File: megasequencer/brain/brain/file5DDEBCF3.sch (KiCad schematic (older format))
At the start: 4 parts

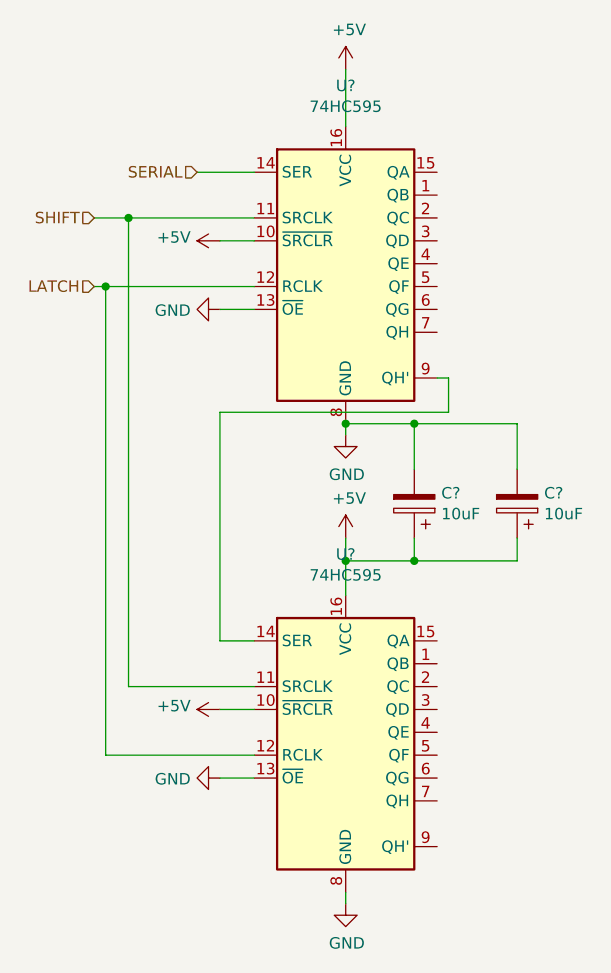
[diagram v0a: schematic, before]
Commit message: Fiddling with PCB a bit
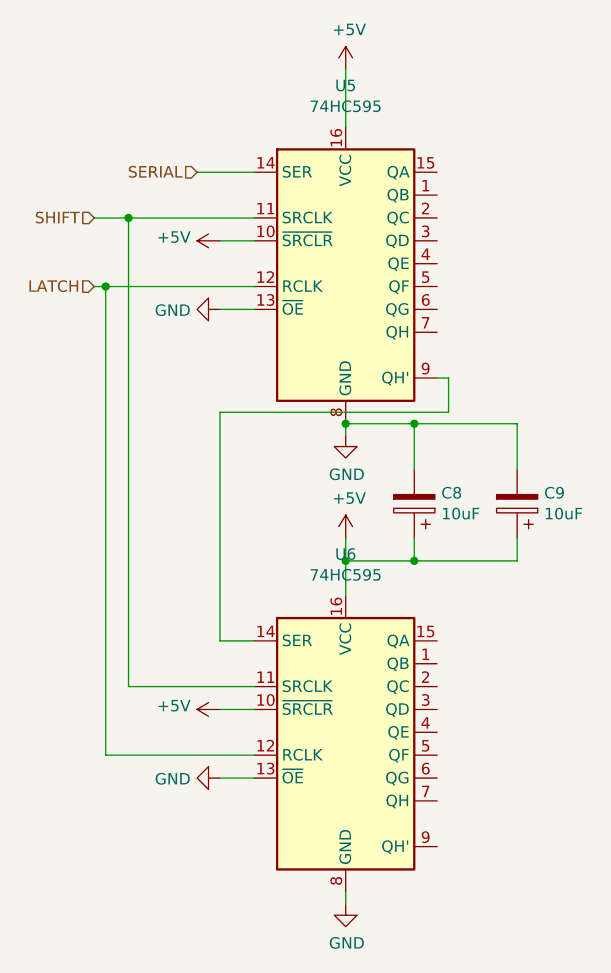
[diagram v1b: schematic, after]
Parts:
- gave numbers to parts that had none: 4
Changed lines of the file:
@@
 $EndDescr
 $Comp
-L power:+5V #PWR?
+L power:+5V #PWR0101
 U 1 1 5DDEC4E8
 P 2300 2150
-F 0 "#PWR?" H 2300 2000 50  0001 C CNN
+F 0 "#PWR0101" H 2300 2000 50  0001 C CNN
 F 1 "+5V" H 2315 2323 50  0000 C CNN
 F 2 "" H 2300 2150 50  0001 C CNN
@@
 $EndComp
 $Comp
-L 74xx:74HC595 U?
+L 74xx:74HC595 U5
 U 1 1 5DDEC62E
 P 2300 3000
-F 0 "U?" H 2300 3778 50  0000 C CNN
+F 0 "U5" H 2300 3778 50  0000 C CNN
 F 1 "74HC595" H 2300 3687 50  0000 C CNN
 F 2 "Package_DIP:DIP-16_W7.62mm" H 2300 3000 50  0001 C CNN
@@
 $EndComp
 $Comp
-L 74xx:74HC595 U?
+L 74xx:74HC595 U6
 U 1 1 5DDEC733
 P 2300 5050
-F 0 "U?" H 2300 5828 50  0000 C CNN
+F 0 "U6" H 2300 5828 50  0000 C CNN
 F 1 "74HC595" H 2300 5737 50  0000 C CNN
 F 2 "Package_DIP:DIP-16_W7.62mm" H 2300 5050 50  0001 C CNN
@@
 	2300 2150 2300 2400
 $Comp
-L power:+5V #PWR?
+L power:+5V #PWR0102
 U 1 1 5DDEC7AF
 P 2300 4200
-F 0 "#PWR?" H 2300 4050 50  0001 C CNN
+F 0 "#PWR0102" H 2300 4050 50  0001 C CNN
 F 1 "+5V" H 2315 4373 50  0000 C CNN
 F 2 "" H 2300 4200 50  0001 C CNN
@@
 	2300 4200 2300 4300
 $Comp
-L power:GND #PWR?
+L power:GND #PWR0103
 U 1 1 5DDEC816
 P 2300 3750
-F 0 "#PWR?" H 2300 3500 50  0001 C CNN
+F 0 "#PWR0103" H 2300 3500 50  0001 C CNN
 F 1 "GND" H 2305 3577 50  0000 C CNN
 F 2 "" H 2300 3750 50  0001 C CNN
@@
 $EndComp
 $Comp
-L power:GND #PWR?
+L power:GND #PWR0104
 U 1 1 5DDEC82E
 P 2300 5800
-F 0 "#PWR?" H 2300 5550 50  0001 C CNN
+F 0 "#PWR0104" H 2300 5550 50  0001 C CNN
 F 1 "GND" H 2305 5627 50  0000 C CNN
 F 2 "" H 2300 5800 50  0001 C CNN
@@
 P 2600 4050
 AR Path="/5E3019D8/5DDED53C" Ref="C?"  Part="1"
-AR Path="/5DDEBCF4/5DDED53C" Ref="C?"  Part="1"
-F 0 "C?" H 2482 4004 50  0000 R CNN
+AR Path="/5DDEBCF4/5DDED53C" Ref="C8"  Part="1"
+F 0 "C8" H 2482 4004 50  0000 R CNN
 F 1 "10uF" H 2482 4095 50  0000 R CNN
 F 2 "Capacitor_THT:CP_Radial_D5.0mm_P2.00mm" H 2638 3900 50  0001 C CNN
@@
 P 3050 4050
 AR Path="/5E3019D8/5DDED5A8" Ref="C?"  Part="1"
-AR Path="/5DDEBCF4/5DDED5A8" Ref="C?"  Part="1"
-F 0 "C?" H 2932 4004 50  0000 R CNN
+AR Path="/5DDEBCF4/5DDED5A8" Ref="C9"  Part="1"
+F 0 "C9" H 2932 4004 50  0000 R CNN
 F 1 "10uF" H 2932 4095 50  0000 R CNN
 F 2 "Capacitor_THT:CP_Radial_D5.0mm_P2.00mm" H 3088 3900 50  0001 C CNN
@@
 Connection ~ 2600 4300
 $Comp
-L power:+5V #PWR?
+L power:+5V #PWR0105
 U 1 1 5DDEDEA1
 P 1750 2900
-F 0 "#PWR?" H 1750 2750 50  0001 C CNN
+F 0 "#PWR0105" H 1750 2750 50  0001 C CNN
 F 1 "+5V" V 1765 3028 50  0000 L CNN
 F 2 "" H 1750 2900 50  0001 C CNN
@@
 $EndComp
 $Comp
-L power:+5V #PWR?
+L power:+5V #PWR0106
 U 1 1 5DDEDEC0
 P 1750 4950
-F 0 "#PWR?" H 1750 4800 50  0001 C CNN
+F 0 "#PWR0106" H 1750 4800 50  0001 C CNN
 F 1 "+5V" V 1765 5078 50  0000 L CNN
 F 2 "" H 1750 4950 50  0001 C CNN
@@
 	1750 4950 1900 4950
 $Comp
-L power:GND #PWR?
+L power:GND #PWR0107
 U 1 1 5DDEE044
 P 1750 3200
-F 0 "#PWR?" H 1750 2950 50  0001 C CNN
+F 0 "#PWR0107" H 1750 2950 50  0001 C CNN
 F 1 "GND" V 1755 3072 50  0000 R CNN
 F 2 "" H 1750 3200 50  0001 C CNN
@@
 	1750 3200 1900 3200
 $Comp
-L power:GND #PWR?
+L power:GND #PWR0108
 U 1 1 5DDEE142
 P 1750 5250
-F 0 "#PWR?" H 1750 5000 50  0001 C CNN
+F 0 "#PWR0108" H 1750 5000 50  0001 C CNN
 F 1 "GND" V 1755 5122 50  0000 R CNN
 F 2 "" H 1750 5250 50  0001 C CNN
